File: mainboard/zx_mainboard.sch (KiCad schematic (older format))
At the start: 93 parts, among them P1 CONN_02X17, P2 CONN_02X20, P3 CONN_02X20, P4 CONN_01X02, Q1 BSS123, Q2 BSS123, Q3 BSS123, Q4 BSS123, Q5 BSS123, Q6 BSS123, Q7 BSS123, Q8 BSS123, U1 4066, U2 4066, U3 4066, U4 4066, U5 4066, U6 74HC14, U7 74HC14

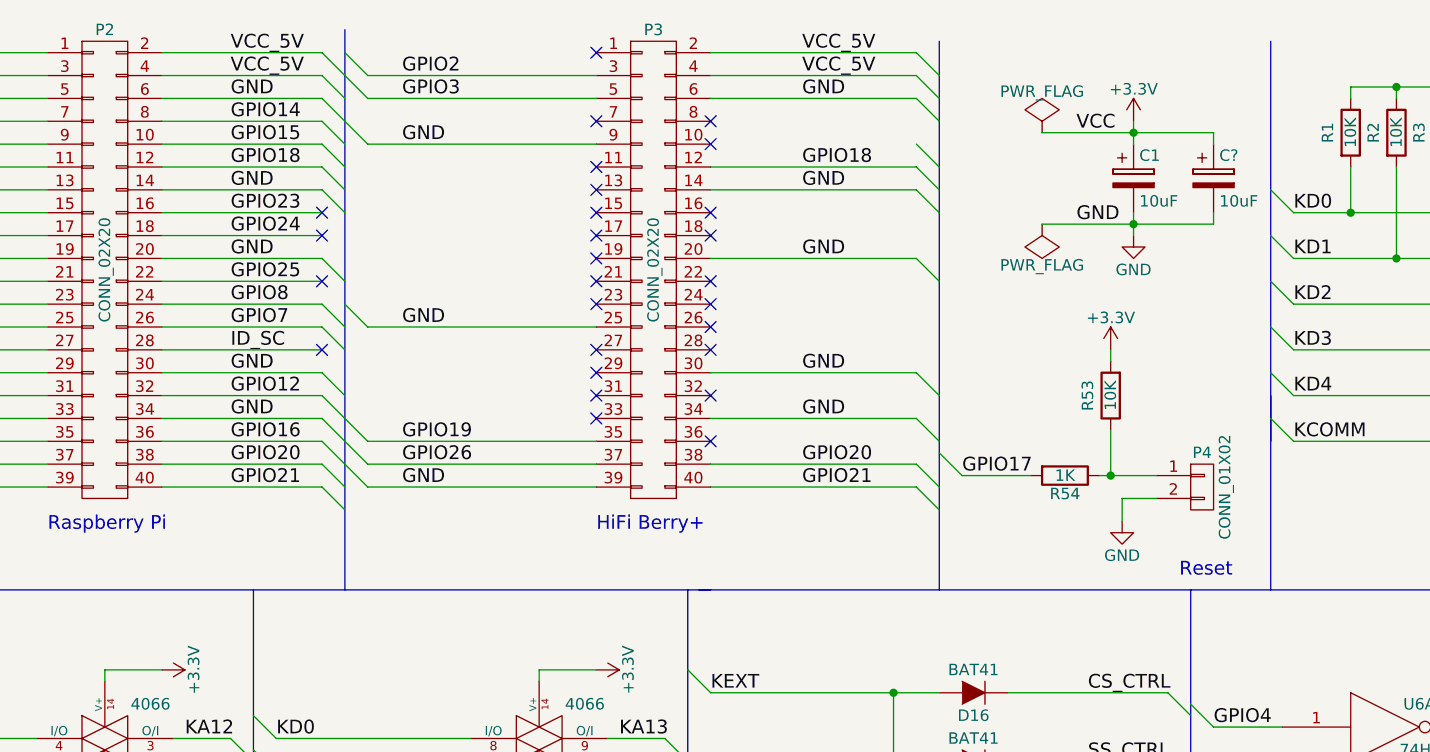
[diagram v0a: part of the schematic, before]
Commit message: pcb
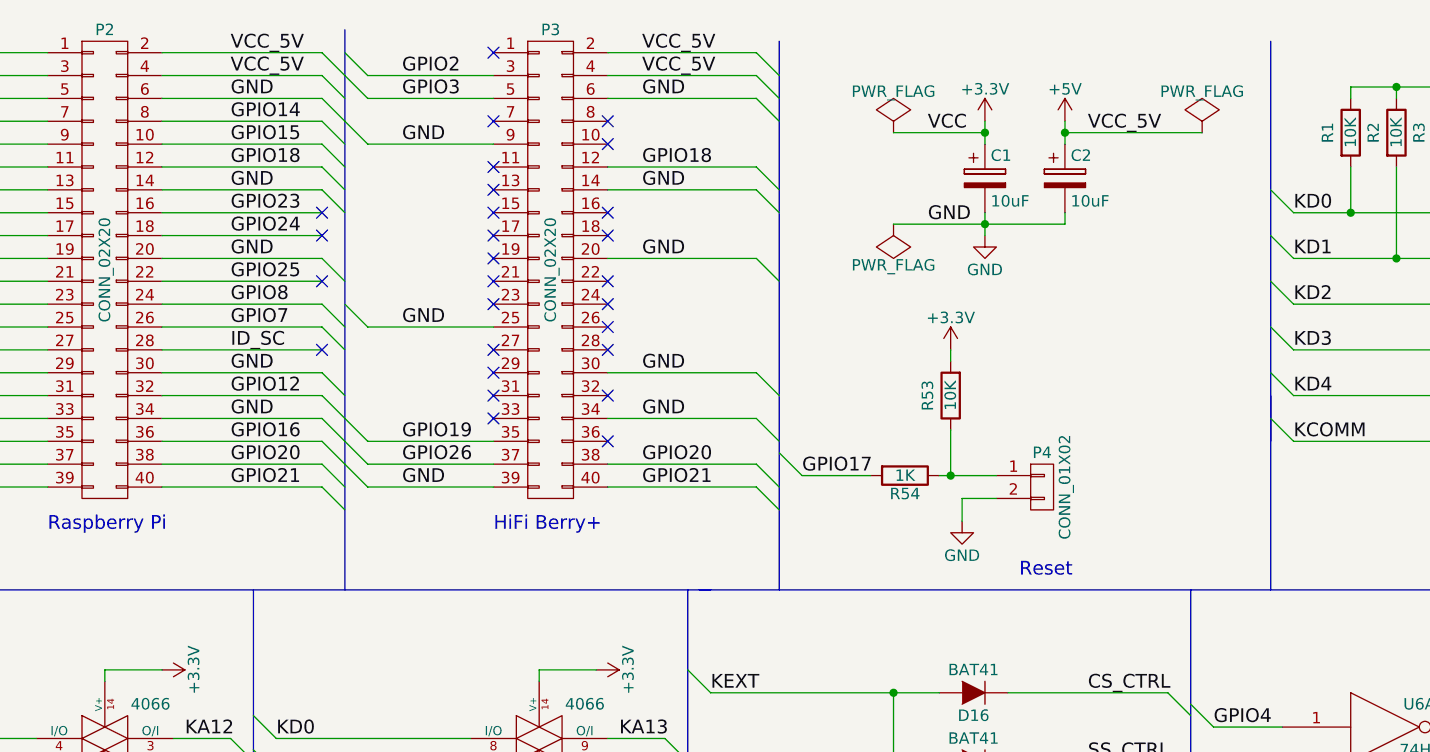
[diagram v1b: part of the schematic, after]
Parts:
- gave numbers to parts that had none: 1
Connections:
- net +3V3: no longer C2.1
- net VCC_5V renamed +5V
- net +5V: now also C2.1
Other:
- moved on the sheet: C1, C2, P3, P4, R53, R54
